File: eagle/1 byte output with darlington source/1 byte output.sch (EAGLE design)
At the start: 8 parts, among them IC1 74LS595N, IC2 74LS595N, X1 MKDSN1,5/9-5,08, X2 MKDSN1,5/8-5,08, X3 MKDSN1,5/5-5,08, X4 MKDSN1,5/5-5,08

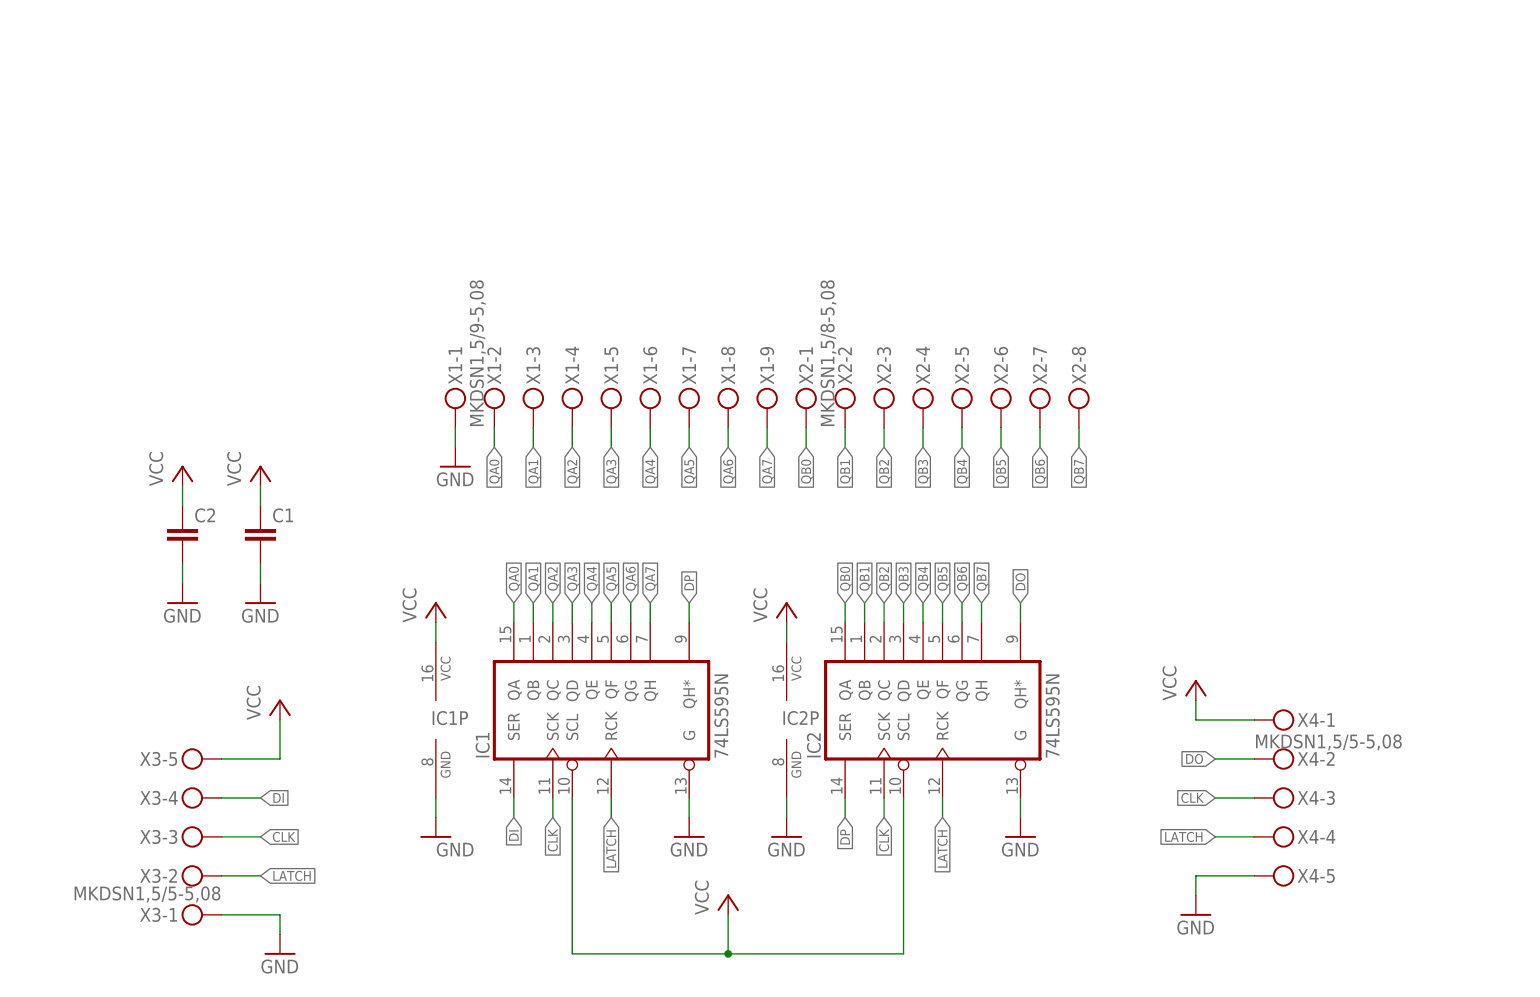
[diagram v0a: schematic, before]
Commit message: periodic check-in
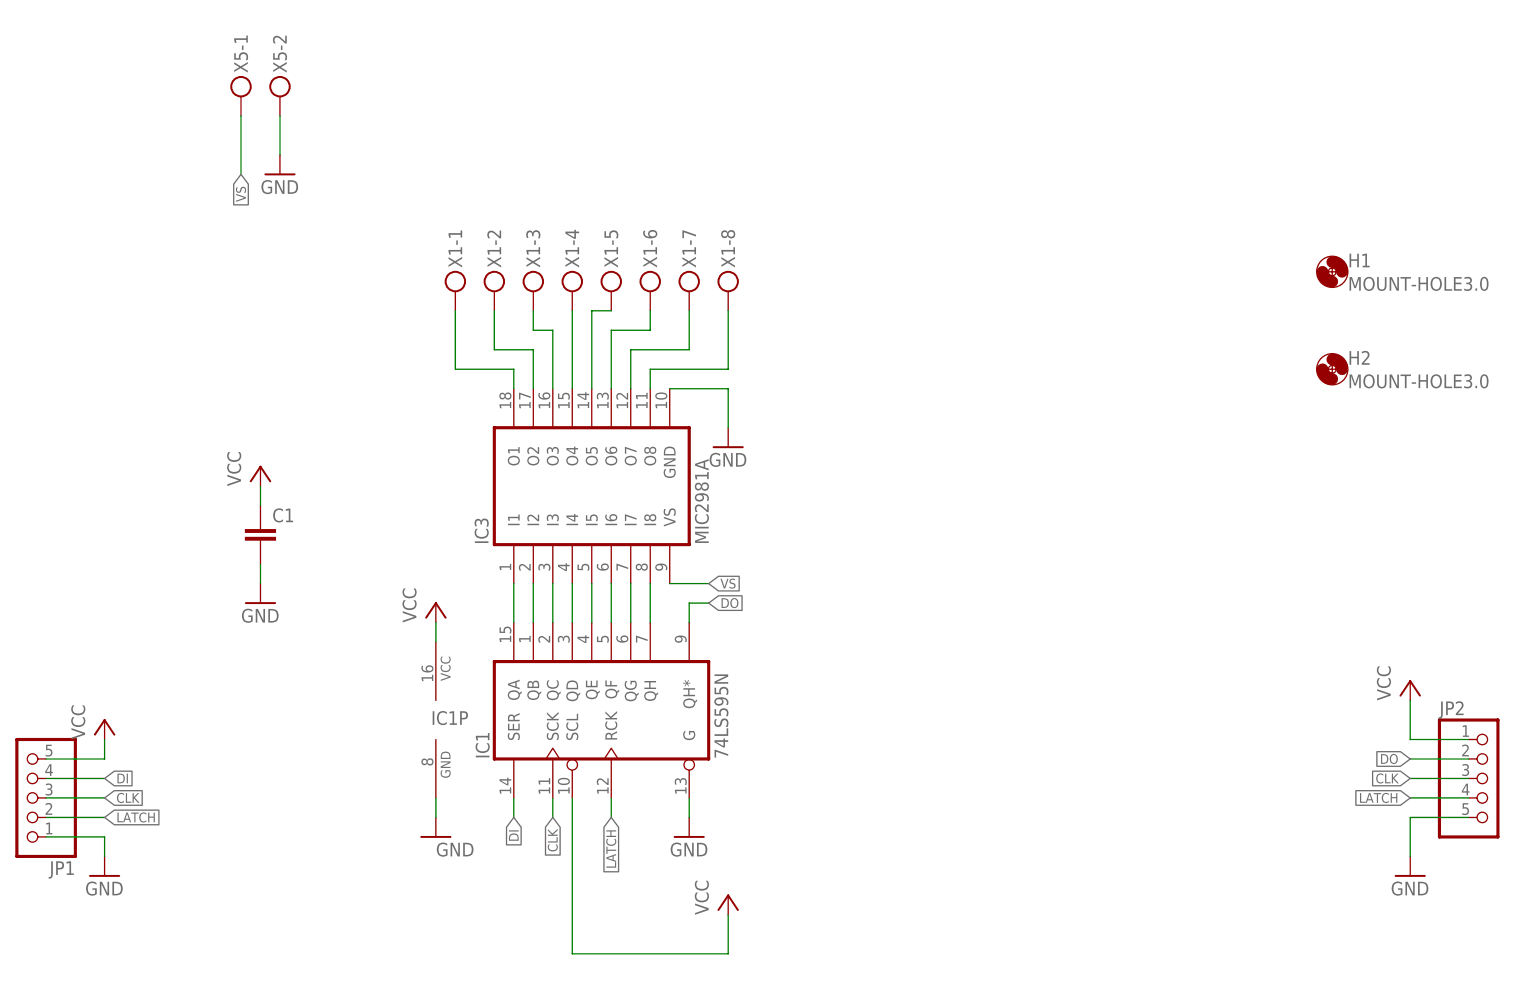
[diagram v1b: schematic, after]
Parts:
- removed C2: (no value), resistor:C-EU050-035X075
- removed IC2: 74LS595N, 74xx-us:74LS595N
- removed X2: MKDSN1,5/8-5,08, con-phoenix-508:MKDSN1,5/8-5,08
- removed X3, X4: MKDSN1,5/5-5,08, con-phoenix-508:MKDSN1,5/5-5,08
- added H1, H2: MOUNT-HOLE3.0, holes:MOUNT-HOLE3.0
- added IC3: MIC2981A, uln-udn:UDN2981A
- added JP1, JP2: (no value), pinhead:PINHD-1X5/90
- added X5: MKDSN1,5/2-5,08, con-phoenix-508:MKDSN1,5/2-5,08
- X1: value MKDSN1,5/9-5,08 -> MKDSN1,5/8-5,08; device con-phoenix-508:MKDSN1,5/9-5,08 -> con-phoenix-508:MKDSN1,5/8-5,08
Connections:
- removed net DP: IC1A.QH*, IC2A.SER
- removed net QA0: IC1A.QA, X1-2.KL
- removed net QA1: IC1A.QB, X1-3.KL
- removed net QA2: IC1A.QC, X1-4.KL
- removed net QA3: IC1A.QD, X1-5.KL
- removed net QA4: IC1A.QE, X1-6.KL
- removed net QA5: IC1A.QF, X1-7.KL
- removed net QA6: IC1A.QG, X1-8.KL
- removed net QA7: IC1A.QH, X1-9.KL
- removed net QB0: IC2A.QA, X2-1.KL
- removed net QB1: IC2A.QB, X2-2.KL
- removed net QB2: IC2A.QC, X2-3.KL
- removed net QB3: IC2A.QD, X2-4.KL
- removed net QB4: IC2A.QE, X2-5.KL
- removed net QB5: IC2A.QF, X2-6.KL
- removed net QB6: IC2A.QG, X2-7.KL
- removed net QB7: IC2A.QH, X2-8.KL
- new net N$1: IC3.O4, X1-4.KL
- new net N$17: IC1A.QA, IC3.I1
- new net N$18: IC1A.QB, IC3.I2
- new net N$19: IC1A.QC, IC3.I3
- new net N$2: IC3.O3, X1-3.KL
- new net N$20: IC1A.QD, IC3.I4
- new net N$21: IC1A.QE, IC3.I5
- new net N$22: IC1A.QF, IC3.I6
- new net N$23: IC1A.QG, IC3.I7
- new net N$24: IC1A.QH, IC3.I8
- new net N$3: IC3.O2, X1-2.KL
- new net N$4: IC3.O1, X1-1.KL
- new net N$5: IC3.O5, X1-5.KL
- new net N$6: IC3.O7, X1-7.KL
- new net N$7: IC3.O8, X1-8.KL
- new net N$8: IC3.O6, X1-6.KL
- new net VS: IC3.VS, X5-1.KL
- net CLK: now also JP1.3, JP2.3; no longer IC2A.SCK, X3-3.KL, X4-3.KL
- net DI: now also JP1.4; no longer X3-4.KL
- net DO: now also IC1A.QH*, JP2.2; no longer IC2A.QH*, X4-2.KL
- net GND: now also IC3.GND, JP1.1, JP2.5, X5-2.KL; no longer C2.2, IC2A.G, IC2P.GND, X1-1.KL, X3-1.KL, X4-5.KL
- net LATCH: now also JP1.2, JP2.4; no longer IC2A.RCK, X3-2.KL, X4-4.KL
- net VCC: now also JP1.5, JP2.1; no longer C2.1, IC2A.SCL, IC2P.VCC, X3-5.KL, X4-1.KL
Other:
- moved on the sheet: X1-1, X1-2, X1-3, X1-4, X1-5, X1-6, X1-7, X1-8
